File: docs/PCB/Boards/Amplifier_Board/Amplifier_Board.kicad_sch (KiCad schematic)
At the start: 46 parts, among them J1 Conn_01x06_Pin, J2 SPEAKER, U1 MCP6002-xSN, U2 LM393, U3 LM386

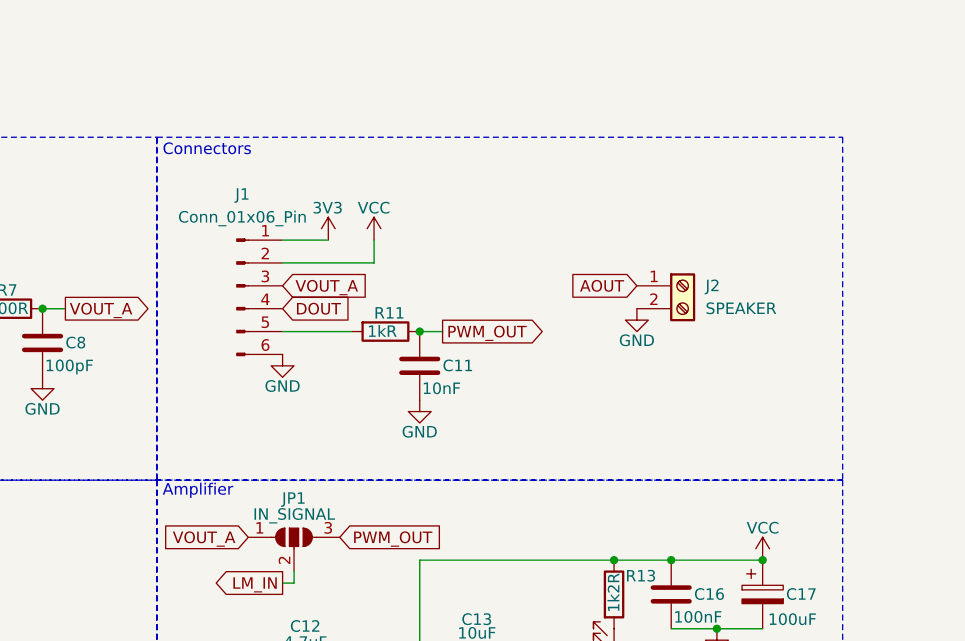
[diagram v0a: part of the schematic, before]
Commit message: Code review
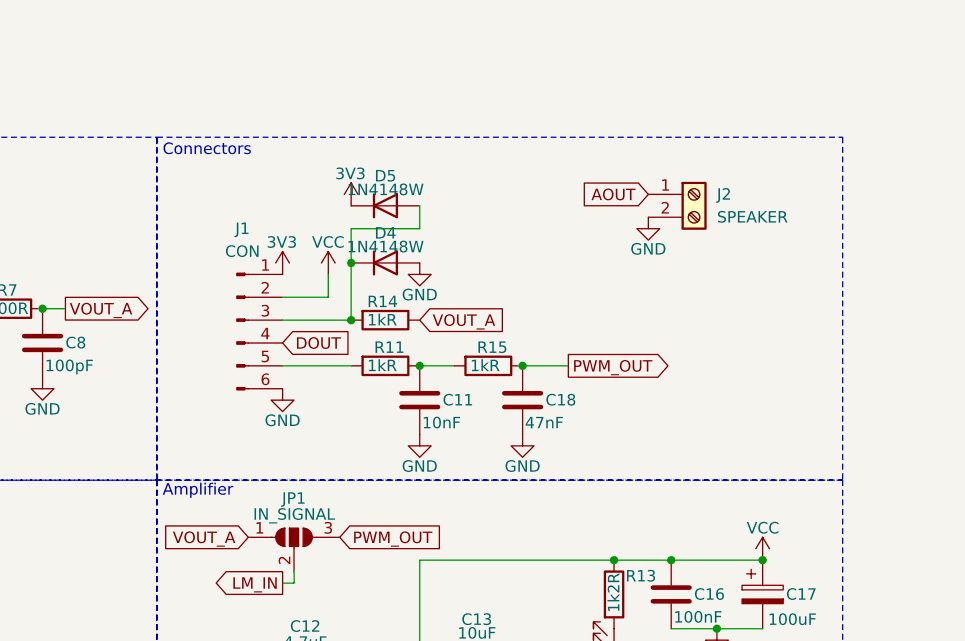
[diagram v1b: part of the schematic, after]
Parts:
- added C18: 47nF, Capacitor_SMD:C_0805_2012Metric, symbol Device:C
- added D4, D5: 1N4148W, Diode_SMD:D_SOD-123, symbol Diode:1N4148W
- added R14, R15: 1kR, Resistor_SMD:R_0805_2012Metric, symbol Device:R
- J1: value Conn_01x06_Pin -> CON
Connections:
- net 3V3: now also D5.1 (K)
- net GND: now also C18.2, D4.2 (A)
- net PWM_OUT: now also C18.1, R15.1; no longer C11.1, R11.1
- net VOUT_A: now also R14.1; no longer J1.3 (Pin_3)
- new net: D4.1 (K), D5.2 (A), J1.3 (Pin_3), R14.2
- new net: C11.1, R11.1, R15.2
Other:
- moved on the sheet: C11, J1, J2, R11
